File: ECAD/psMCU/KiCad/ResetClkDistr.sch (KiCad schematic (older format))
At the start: 4 parts, among them U308 SN74LVC1G04DCK, U35 SN74HC245PW

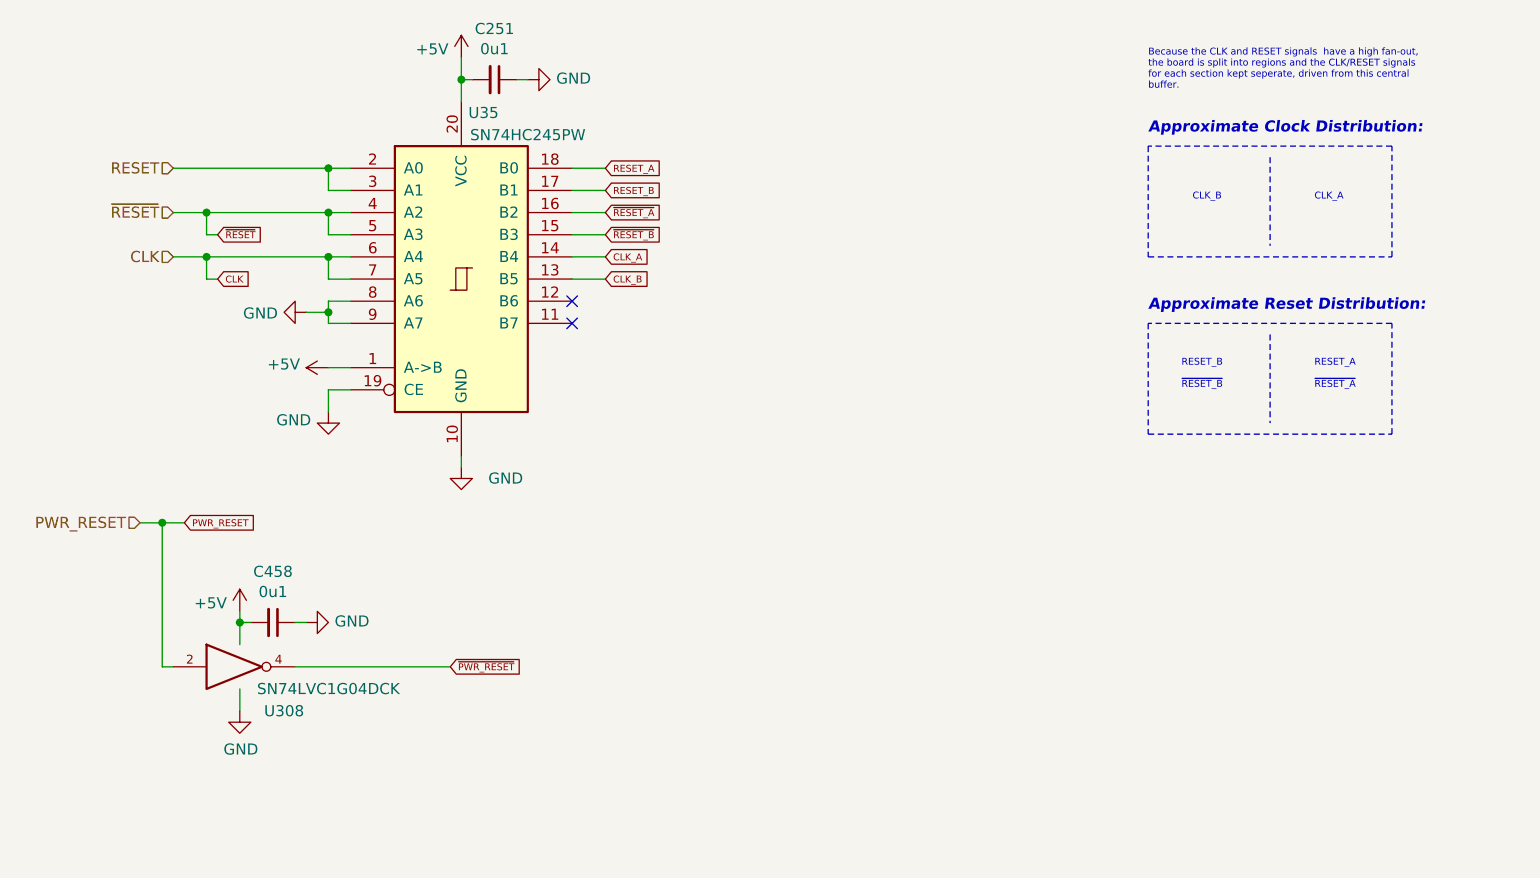
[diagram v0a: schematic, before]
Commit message: Sch: Cleanup + Small fixes
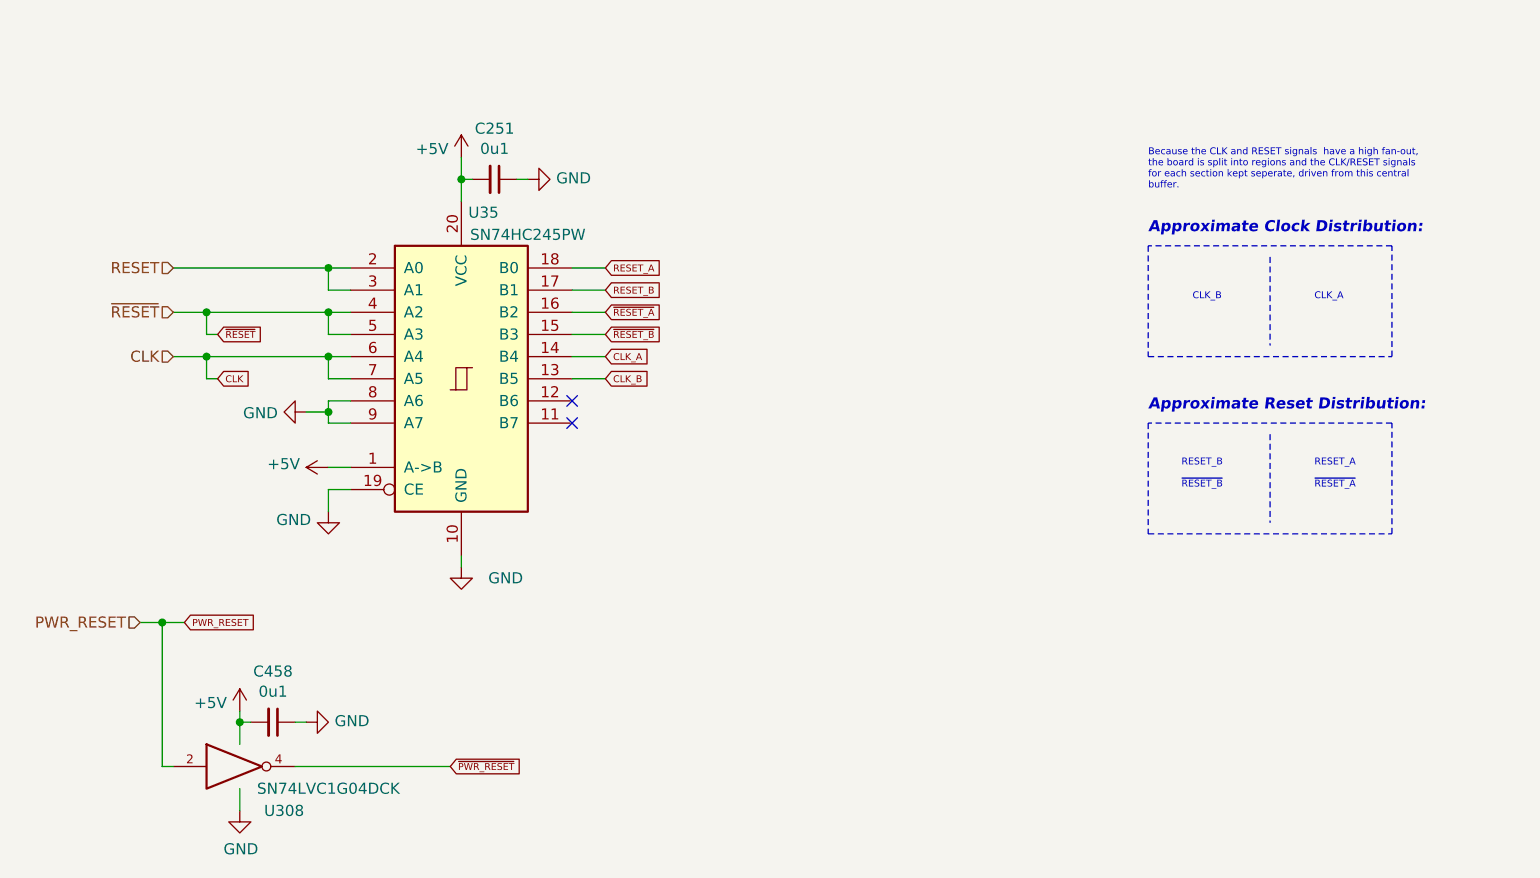
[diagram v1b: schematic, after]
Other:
- moved on the sheet: C251, C458, U308, U35
